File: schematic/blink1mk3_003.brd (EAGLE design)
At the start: 88.5 x 50.8 mm, 36 parts, among them J1 NONPOP, U1 EFM32HG309F64G, X1 USBPCB2, X2 USBPCB2, X3 USBPCB2

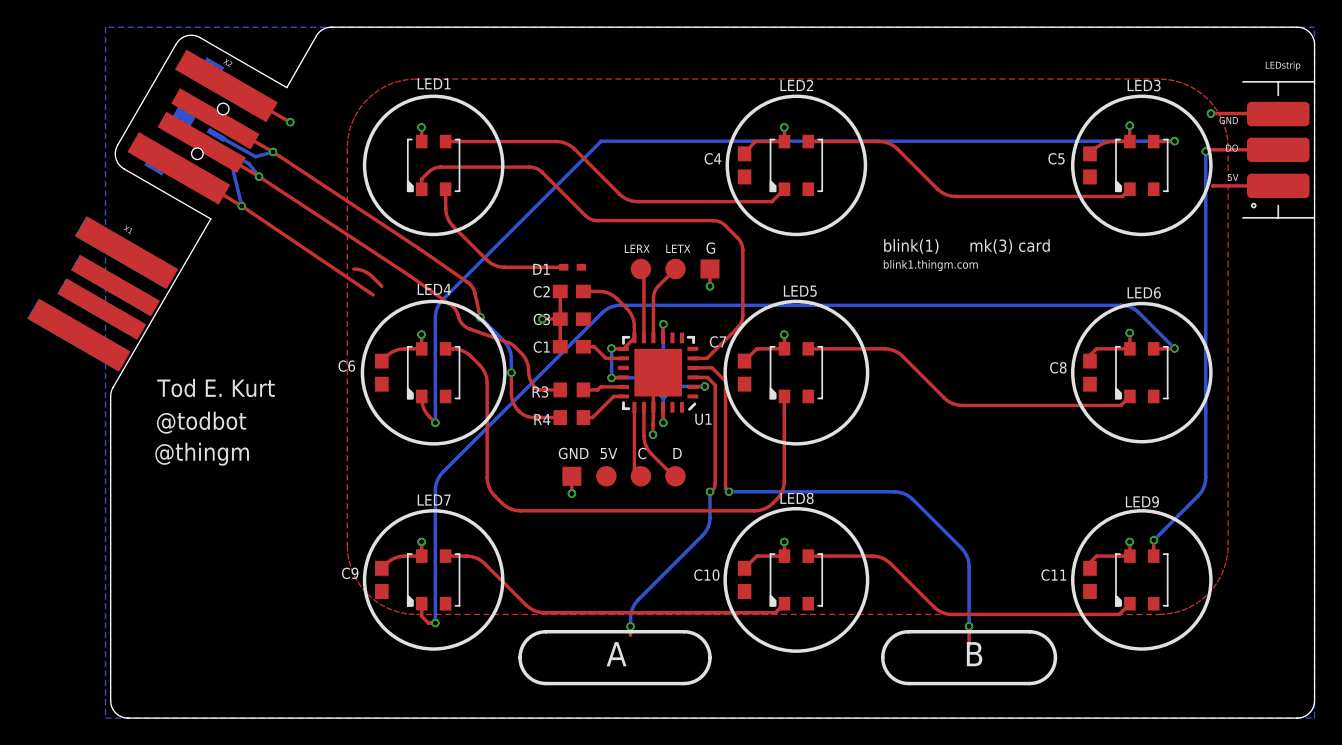
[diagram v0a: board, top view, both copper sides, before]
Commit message: sync schematic experiments
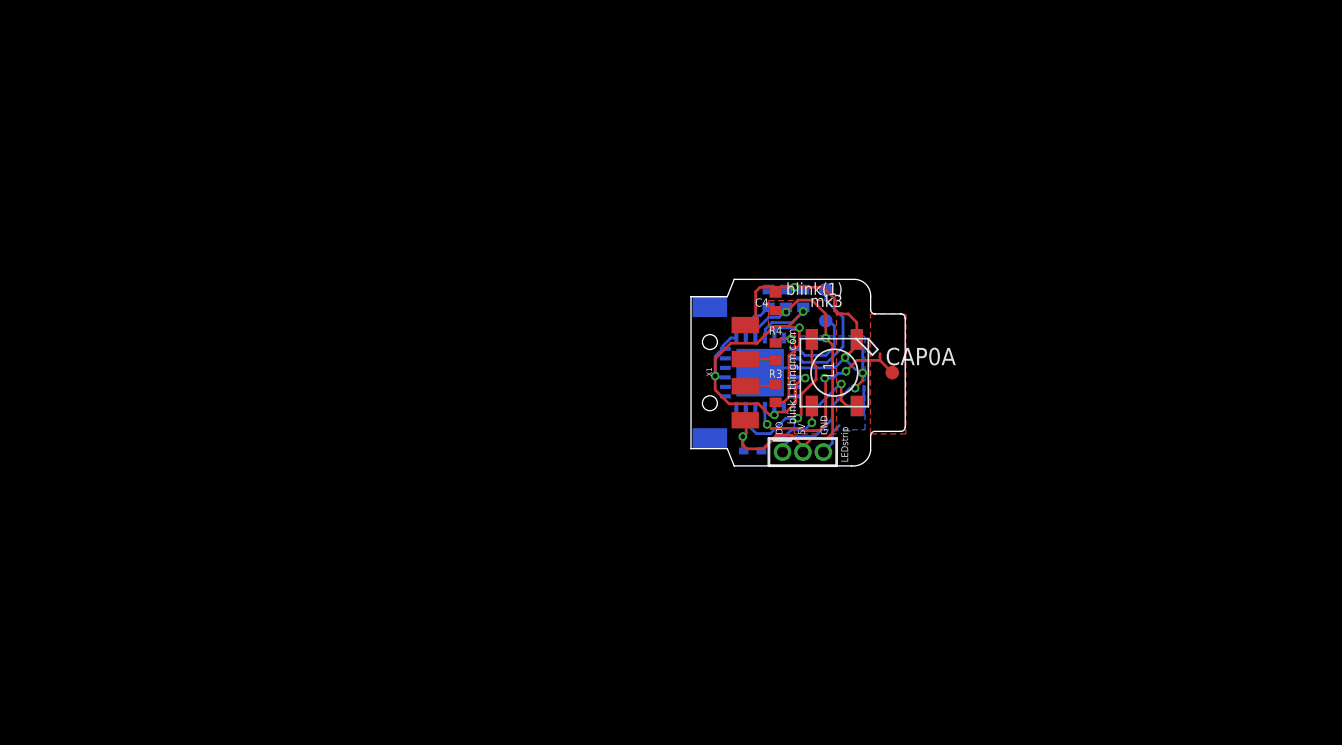
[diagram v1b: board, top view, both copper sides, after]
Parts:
- removed 5V, LERX, LETX: TPTP15R, testpad:TP15R
- removed C10, C11, C5, C6, C7, C8, C9: 0.1uF, adafruit:C0603
- removed G, GND: TPTP14SQ, testpad:TP14SQ
- removed J1: NONPOP, SparkFun-Connectors:USB-B-MICRO-SMD
- removed LED1, LED2, LED3, LED4, LED5, LED6, LED7, LED8, LED9: SK6812MINI, adafruit:LED3535
- removed U$1: LED_STRIP_3P, NeoJoints:LEDSTRIP-3P
- removed X2, X3: USBPCB2, todstuff:USB-A-PCB-2
- added CAP0A: TPTP10R, testpad:TP10R
- added JP3: M03MM, todstuff:1X03-1.5MM
- added L1, L2: WS2812B, adafruit:WS2812B
- C, D: value TPTP15R -> TPTP10R; device testpad:TP15R -> testpad:TP10R
- C1, C2, C3, C4: device adafruit:C0603 -> adafruit:C0402
- R3, R4: device adafruit:R0603 -> adafruit:R0402
- X1: value USBPCB2 -> USB; device todstuff:USB-A-PCB-2 -> todstuff:MOLEX-48037-1000
- moved X1 43.6 mm to (-0.01, 0.00), turned to 0 degrees
- moved D1 19.0 mm to (3.17, -5.76), flipped to the bottom
- moved C 17.8 mm to (8.51, 3.81), flipped to the bottom
- moved D 17.6 mm to (8.51, 6.10), flipped to the bottom
- moved C2 17.0 mm to (6.86, 5.46), flipped to the bottom, turned to 90 degrees
- moved C3 15.8 mm to (5.59, 5.46), flipped to the bottom, turned to 90 degrees
- moved R4 15.7 mm to (4.83, 1.52), turned to 270 degrees
- moved R3 15.0 mm to (4.83, -1.52), turned to 90 degrees
- moved C1 14.9 mm to (4.32, 5.46), flipped to the bottom, turned to 90 degrees
- moved C4 10.3 mm to (4.83, 5.21)
- moved U1 7.49 mm to (3.68, 0.00), flipped to the bottom, turned to 90 degrees
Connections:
- removed net N$10: LED6.3, LED7.1
- removed net N$4: LED7.3, LED8.1
- removed net N$5: LED4.3, LED5.1
- removed net N$6: LED5.3, LED6.1
- removed net N$7: LED2.3, LED3.1
- removed net N$8: LED3.3, LED4.1
- removed net N$9: LED8.3, LED9.1
- removed net VBUS: X1.5V, X3.5V
- net +5V: now also JP3.2, L2.1-VDD, X1.1; no longer 5V.TP, C10.1, C11.1, C5.1, C6.1, C7.1, C8.1, C9.1, J1.VBUS, LED2.2, LED3.2, LED4.2, LED5.2, LED6.2, LED7.2, LED8.2, LED9.2, U$1.A, X2.5V
- net CAP0A: now also CAP0A.TP
- net DI: now also L1.4-DIN; no longer LED1.1
- net DO: now also JP3.1, L2.2-DOUT; no longer LED9.3, U$1.B
- net GND: now also JP3.3, L1.3-GND, L2.3-GND, X1.4; no longer C10.2, C11.2, C5.2, C6.2, C7.2, C8.2, C9.2, G.TP, GND.TP, J1.GND, LED1.4, LED2.4, LED3.4, LED4.4, LED5.4, LED6.4, LED7.4, LED8.4, LED9.4, U$1.C, X1.GND, X2.GND, X3.GND
- net LEUO_RX: no longer LERX.TP
- net LEUO_TX: no longer LETX.TP
- net N$2: now also L1.2-DOUT, L2.4-DIN; no longer LED1.3, LED2.1
- net USB_D+: now also X1.3; no longer J1.D+, X2.USB_P
- net USB_D-: now also X1.2; no longer J1.D-, X2.USB_M
- net VLEDA: now also L1.1-VDD; no longer LED1.2
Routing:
- net N$10: track 74.9 -> 0.00 mm, vias 2 -> 0
- net N$8: track 71.7 -> 0.00 mm, vias 2 -> 0
- net N$5: track 41.7 -> 0.00 mm
- net USB_D+: track 40.5 -> 2.77 mm, vias 3 -> 0
- net CAP1A: track 37.0 -> 0.00 mm, vias 2 -> 0
- net USB_D-: track 37.3 -> 2.77 mm, vias 1 -> 0
- net N$4: track 26.7 -> 0.00 mm
- net N$9: track 25.5 -> 0.00 mm
- net N$6: track 25.4 -> 0.00 mm
- net N$7: track 25.3 -> 0.00 mm
- net GND: track 59.3 -> 34.2 mm, vias 15 -> 2
- net DI: track 37.2 -> 12.2 mm, vias 0 -> 1
- net DO: track 36.6 -> 12.1 mm
- net N$2: track 26.9 -> 5.56 mm, vias 0 -> 1
- net CAP0A: track 22.6 -> 15.8 mm, vias 2 -> 3
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- removed copper zone on layer 1, net CAP1A
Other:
- board size 88.5 x 50.8 mm -> 15.7 x 13.7 mm
- board text added: "blink1mk3_003"
- board text added: "mk3"
- board text removed: "@thingm"
- board text removed: "@todbot"
- board text removed: "A"
- board text removed: "B"
- board text removed: "Tod E. Kurt"
- board text removed: "blink1mk3_card"
- board text removed: "mk(3) card"
